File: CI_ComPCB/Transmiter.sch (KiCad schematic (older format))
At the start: 7 parts, among them J501 RJ45_LED_Shielded, J502 RJ45_LED_Shielded

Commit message: Production1
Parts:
- removed Converter501: TxRx-RS485, CI_ComPCB:TXRX-AB, symbol CI_ComPCB-rescue:TxRx-RS485-New_Library-RackComm-rescue-CI_ComPCB-rescue
- removed D501: SS34, digikey-footprints:DO-214AC, symbol CI_ComPCB-rescue:SS34-SamacSys_Parts
- removed J502: RJ45_LED_Shielded, Connector_RJ:RJ45_Amphenol_RJHSE538X, symbol Connector:RJ45_LED_Shielded
- removed R502: 680, Resistor_SMD:R_0805_2012Metric, symbol Device:R
- Converter301: renamed from Converter502; symbol CI_ComPCB-rescue:TxRx-RS485-New_Library-RackComm-rescue-CI_ComPCB-rescue -> CI_ComPCB-rescue:TxRx-RS485-New_Library-RackComm-rescue-CI_ComPCB-rescue-CI_ComPCB-rescue
- renumbered J501 to J301, R501 to R301
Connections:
- net labels removed: A0, B0, RX0, RX1, Sheild, TX0, TX1
- wire segments 49 -> 18
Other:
- moved on the sheet: J301, R301

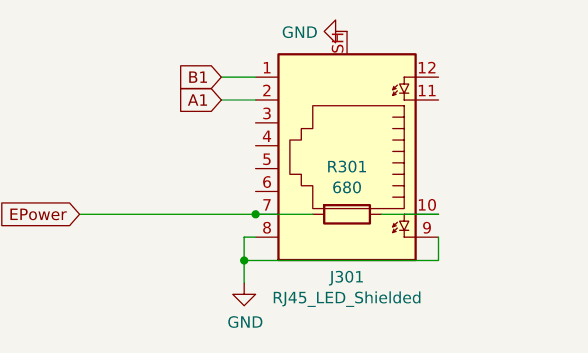
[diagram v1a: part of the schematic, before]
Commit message: prilim pcb finished
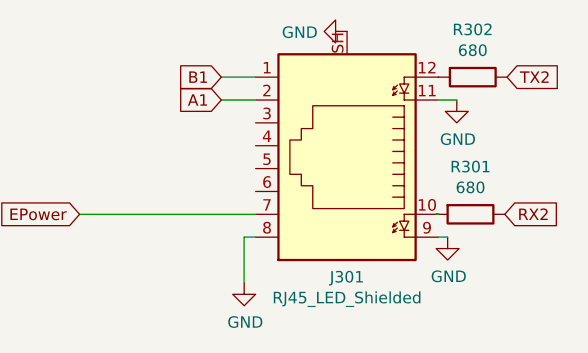
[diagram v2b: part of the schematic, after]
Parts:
- added R302: 680, Resistor_SMD:R_0805_2012Metric, symbol Device:R
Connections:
- net EPower: no longer R301.2
- net GND: now also J301.11
- net RX2: now also R301.1
- net TX2: now also R302.1
- net at J301.10: now also R301.2; no longer R301.1
- net at J301.12: now also R302.2
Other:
- moved on the sheet: R301
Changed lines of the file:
@@
 L Device:R R?
 U 1 1 61AB18D1
-P 7400 5140
+P 7940 5140
 AR Path="/61AB18D1" Ref="R?"  Part="1"
 AR Path="/61A9C8FD/61AB18D1" Ref="R301"  Part="1"
-F 0 "R301" V 7193 5140 50  0000 C CNN
-F 1 "680" V 7284 5140 50  0000 C CNN
-F 2 "Resistor_SMD:R_0805_2012Metric" V 7330 5140 50  0001 C CNN
-F 3 "~" H 7400 5140 50  0001 C CNN
-	1    7400 5140
+F 0 "R301" V 7733 5140 50  0000 C CNN
+F 1 "680" V 7824 5140 50  0000 C CNN
+F 2 "Resistor_SMD:R_0805_2012Metric" V 7870 5140 50  0001 C CNN
+F 3 "~" H 7940 5140 50  0001 C CNN
+	1    7940 5140
 	0    1    1    0
 $EndComp
-Wire Wire Line
-	6950 5240 6950 5342
 $Comp
 L power:GND #PWR?
@@
 $EndComp
 Wire Wire Line
-	7550 5140 7800 5140
-Wire Wire Line
 	7000 4640 6850 4640
 Wire Wire Line
@@
 Wire Wire Line
 	6950 5240 7000 5240
-Wire Wire Line
-	7800 5240 7800 5342
-Wire Wire Line
-	7800 5342 6950 5342
-Connection ~ 6950 5342
-Wire Wire Line
-	6950 5342 6950 5440
-Connection ~ 7000 5140
-Wire Wire Line
-	7000 5140 7250 5140
-Wire Wire Line
-	6230 5140 7000 5140
 $Comp
 L Connector:RJ45_LED_Shielded J?
@@
 	-1   0    0    1
 $EndComp
+$Comp
+L Device:R R?
+U 1 1 626CFBAF
+P 7950 4540
+AR Path="/626CFBAF" Ref="R?"  Part="1"
+AR Path="/61A9C8FD/626CFBAF" Ref="R302"  Part="1"
+F 0 "R302" V 7743 4540 50  0000 C CNN
+F 1 "680" V 7834 4540 50  0000 C CNN
+F 2 "Resistor_SMD:R_0805_2012Metric" V 7880 4540 50  0001 C CNN
+F 3 "~" H 7950 4540 50  0001 C CNN
+	1    7950 4540
+	0    1    1    0
+$EndComp
+$Comp
+L power:GND #PWR?
+U 1 1 626D253E
+P 7880 4640
+AR Path="/626D253E" Ref="#PWR?"  Part="1"
+AR Path="/61A9C8FD/626D253E" Ref="#PWR0106"  Part="1"
+F 0 "#PWR0106" H 7880 4390 50  0001 C CNN
+F 1 "GND" H 7885 4467 50  0000 C CNN
+F 2 "" H 7880 4640 50  0001 C CNN
+F 3 "" H 7880 4640 50  0001 C CNN
+	1    7880 4640
+	1    0    0    -1
+$EndComp
+Wire Wire Line
+	7800 4640 7880 4640
+Wire Wire Line
+	7800 5240 7840 5240
+Wire Wire Line
+	6230 5140 7000 5140
+Wire Wire Line
+	6950 5240 6950 5440
+Wire Wire Line
+	7790 5140 7800 5140
+$Comp
+L power:GND #PWR?
+U 1 1 626DB77D
+P 7840 5240
+AR Path="/626DB77D" Ref="#PWR?"  Part="1"
+AR Path="/61A9C8FD/626DB77D" Ref="#PWR0107"  Part="1"
+F 0 "#PWR0107" H 7840 4990 50  0001 C CNN
+F 1 "GND" H 7845 5067 50  0000 C CNN
+F 2 "" H 7840 5240 50  0001 C CNN
+F 3 "" H 7840 5240 50  0001 C CNN
+	1    7840 5240
+	1    0    0    -1
+$EndComp
+Text GLabel 8100 4540 2    50   Input ~ 0
+TX2
+Text GLabel 8090 5140 2    50   Input ~ 0
+RX2
 $EndSCHEMATC
